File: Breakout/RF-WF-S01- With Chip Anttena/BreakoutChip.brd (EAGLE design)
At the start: 43.7 x 25.9 mm, 61 parts, among them U2 FT2232D, U3 LMR10510XMFE, U5 93LC46BT-I/OT

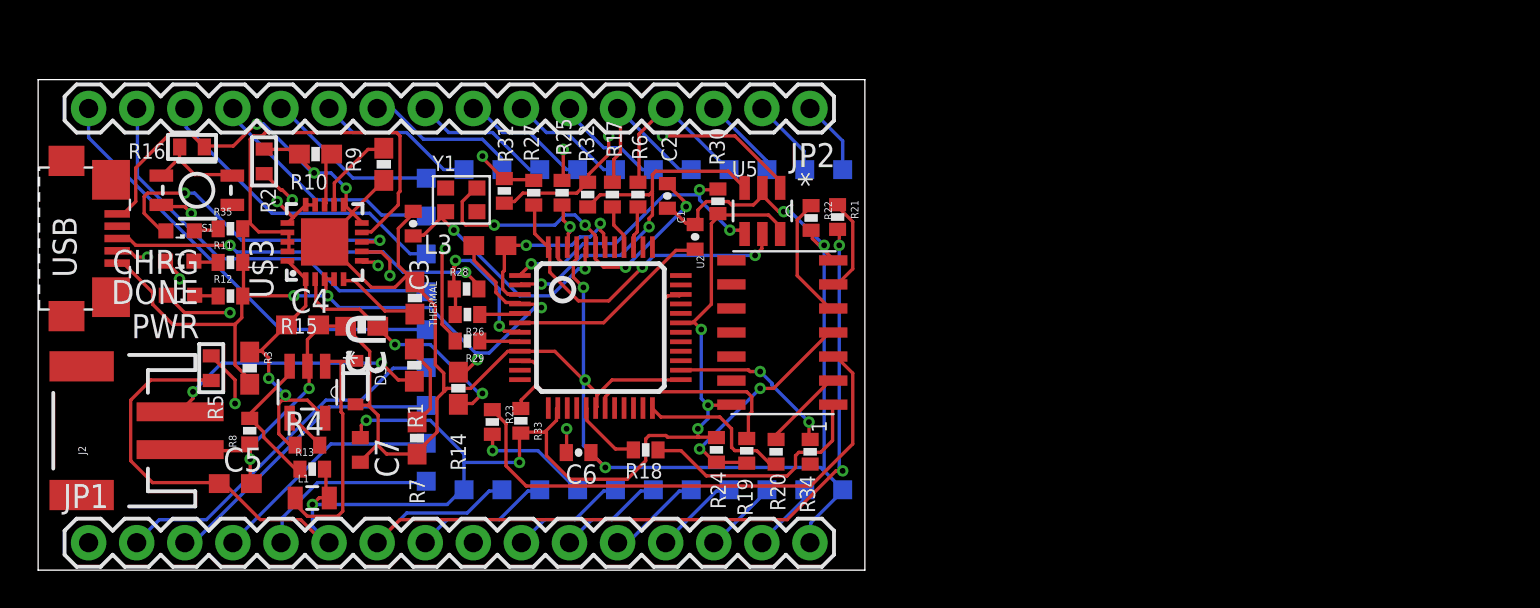
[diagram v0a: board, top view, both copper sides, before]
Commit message: Some cleanup
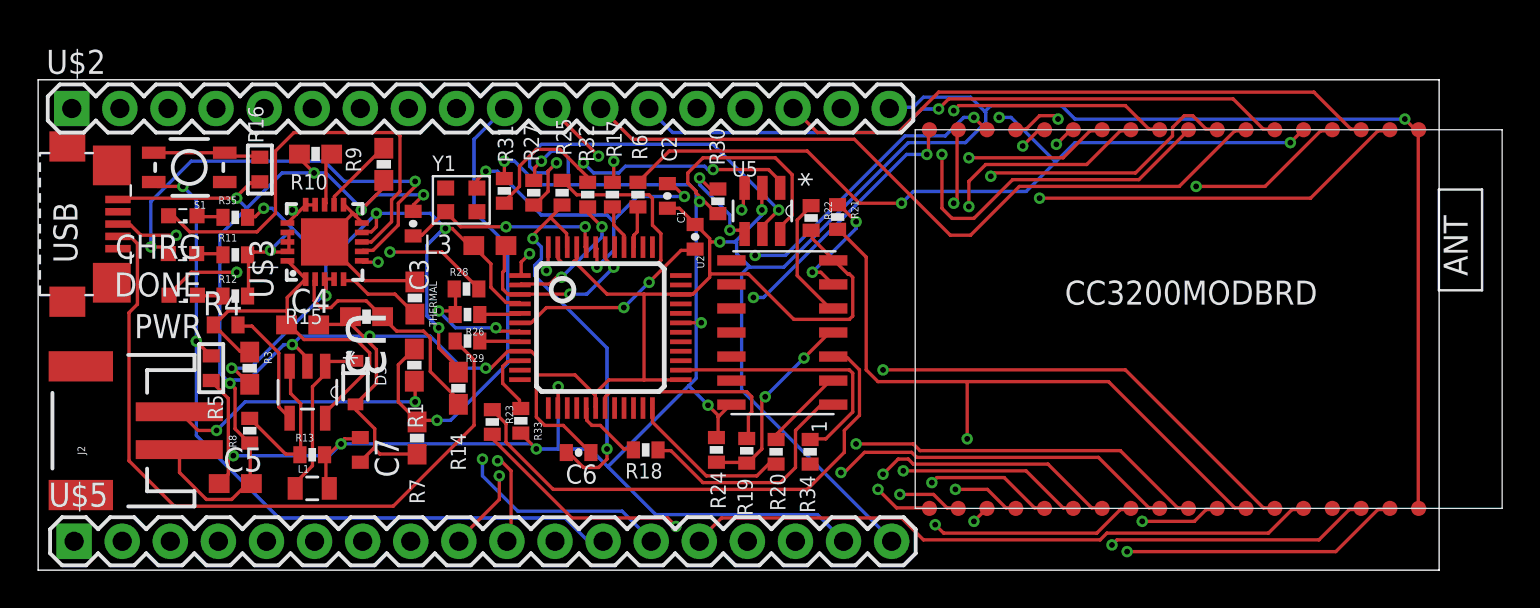
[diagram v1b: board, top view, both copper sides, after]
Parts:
- removed JP1, JP2: M16PTH, DECADE-libraries:1X16
- removed R2: (no value), microbuilder:0402
- added U$2, U$5: M18_, DECADE-libraries:1X18
- U$1: value WEBEE_WIFI_CC3200 -> CC3200MOD; device WeeBee:CC3200 -> CC3200MODBRD:CC3200MOD
- moved U$1 30.3 mm to (61.8, 13.3), flipped to the top, turned to 0 degrees
- moved R4 7.68 mm to (9.91, 13.0)
- moved R16 3.78 mm to (11.7, 21.2), turned to 90 degrees
- moved S1 1.27 mm to (7.98, 21.3)
- moved CHRG 0.81 mm to (7.64, 18.7)
- moved USB 0.76 mm to (1.54, 18.3)
- moved R13 0.76 mm to (14.5, 6.10)
- moved R35 0.65 mm to (10.4, 18.6)
- moved R15 0.57 mm to (17.3, 13.4)
- moved L1 0.51 mm to (14.5, 4.32)
- moved R11 0.47 mm to (10.4, 16.7)
- moved DONE 0.43 mm to (7.62, 16.7)
- moved R12 0.25 mm to (10.4, 14.5)
- moved PWR 0.15 mm to (7.66, 14.5)
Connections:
- removed net G00: JP2.3, U$1.G00
- removed net N$12: JP2.1, U$1.G31
- removed net N$2: JP1.15, U$1.TMS
- removed net N$22: JP2.11, U$1.G08
- removed net N$23: JP2.12, U$1.G09
- removed net N$24: JP1.5, U$1.G17
- removed net N$28: JP2.16, U$1.G13
- removed net N$6: JP1.11, U$1.TDI
- removed net N$7: JP1.10, U$1.G22
- new net N$10: U$1.P04, U$2.11
- new net N$14: U$1.P07/TX, U$2.8
- new net N$15: U$1.P08, U$2.7
- new net N$16: U$1.P09, U$2.6
- new net N$32: U$1.P19/TCK, U$5.8
- new net N$33: U$1.P28, U$5.7
- new net N$34: U$1.P24/TDO, U$5.6
- new net N$35: U$1.P23/TDI, U$5.5
- new net N$36: U$1.P22, U$5.4
- new net N$37: U$1.P17, U$5.3
- new net N$52: U$1.P16, U$5.2
- new net N$53: U$1.P15, U$5.1
- net FTDI_RX: now also U$1.P01, U$2.14; no longer JP2.4, U$1.G01
- net FTDI_TX: now also U$1.P02, U$2.13; no longer JP2.5, U$1.G02
- net GND: now also U$1.GND1, U$2.18, U$5.18; no longer JP1.16, R2.1
- net GPIO_05: now also U$1.P05, U$2.10
- net N$13: now also U$1.P06, U$2.9; no longer JP2.2, U$1.G30
- net N$17: now also U$1.P10, U$2.5; no longer JP2.6, U$1.G03
- net N$18: now also U$1.P11, U$2.4; no longer JP2.7, U$1.G04
- net N$19: now also U$1.P12, U$2.3; no longer JP2.8, U$1.G05
- net N$20: now also U$1.P13, U$2.2; no longer JP2.9, U$1.G06
- net N$21: now also U$1.P14, U$2.1; no longer JP2.10, U$1.G07
- net N$25: now also U$1.SOP1, U$5.15; no longer JP2.13, U$1.G10
- net N$26: now also U$1.SOP0, U$5.14; no longer JP2.14, U$1.G11
- net N$27: now also U$1.P31/RX, U$5.13; no longer JP2.15, U$1.G12
- net N$29: now also U$1.P27, U$5.11; no longer JP1.4, U$1.G16
- net N$3: now also U$1.RFOUT, U$2.17; no longer JP1.14, U$1.TCK
- net N$30: now also U$1.P26, U$5.10; no longer JP1.3, U$1.G15
- net N$31: now also U$1.P29/TMS, U$5.9; no longer JP1.2, U$1.G14
- net N$4: now also U$1.P00, U$2.16; no longer JP1.13, U$1.G28
- net N$5: now also U$1.P30, U$2.15; no longer JP1.12, U$1.TDO
- net N$9: now also U$1.P03, U$2.12; no longer JP1.8, U$1.SOP0
- net RST: now also U$1.RESET, U$5.12; no longer JP1.7, U$1.RST
- net SOP2: now also U$1.P25/SOP2, U$5.16; no longer R2.2, U$1.SOP2
- net VCC: now also U$5.17; no longer JP1.6
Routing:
- net GND: track 154.1 -> 230.1 mm, vias 10 -> 11
- net GPIO_05: track 4.49 -> 67.7 mm, vias 0 -> 2
- net N$14: track 0.00 -> 58.9 mm, vias 0 -> 1
- net FTDI_RX: track 9.29 -> 60.1 mm, vias 0 -> 3
- net N$18: track 6.30 -> 54.2 mm, vias 0 -> 1
- net N$53: track 0.00 -> 46.7 mm, vias 0 -> 1
- net N$20: track 7.40 -> 53.7 mm, vias 0 -> 1
- net N$36: track 0.00 -> 46.2 mm, vias 0 -> 1
- net N$21: track 8.29 -> 54.2 mm, vias 0 -> 2
- net N$52: track 0.00 -> 45.5 mm, vias 0 -> 1
- net N$17: track 5.92 -> 51.2 mm, vias 0 -> 1
- net N$37: track 0.00 -> 44.5 mm, vias 0 -> 1
- net N$35: track 0.00 -> 44.4 mm, vias 0 -> 1
- net N$16: track 0.00 -> 43.5 mm, vias 0 -> 1
- net N$19: track 6.84 -> 49.8 mm, vias 0 -> 2
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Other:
- board size 43.7 x 25.9 mm -> 74 x 25.9 mm
